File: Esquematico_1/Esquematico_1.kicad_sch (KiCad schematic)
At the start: 0 parts

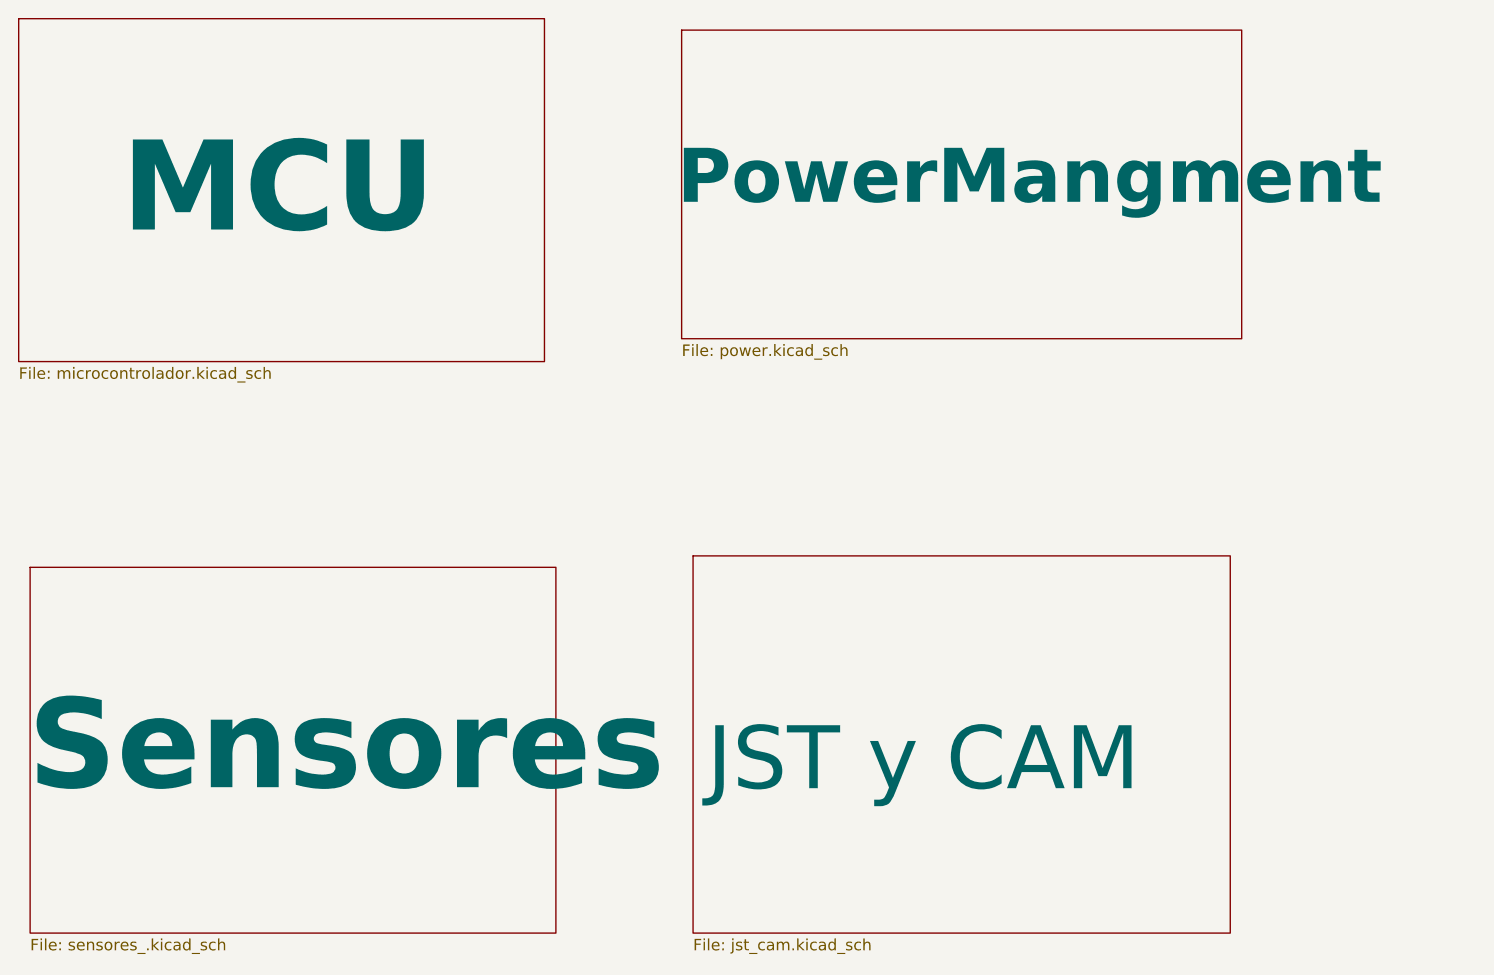
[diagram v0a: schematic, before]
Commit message: Update llamada
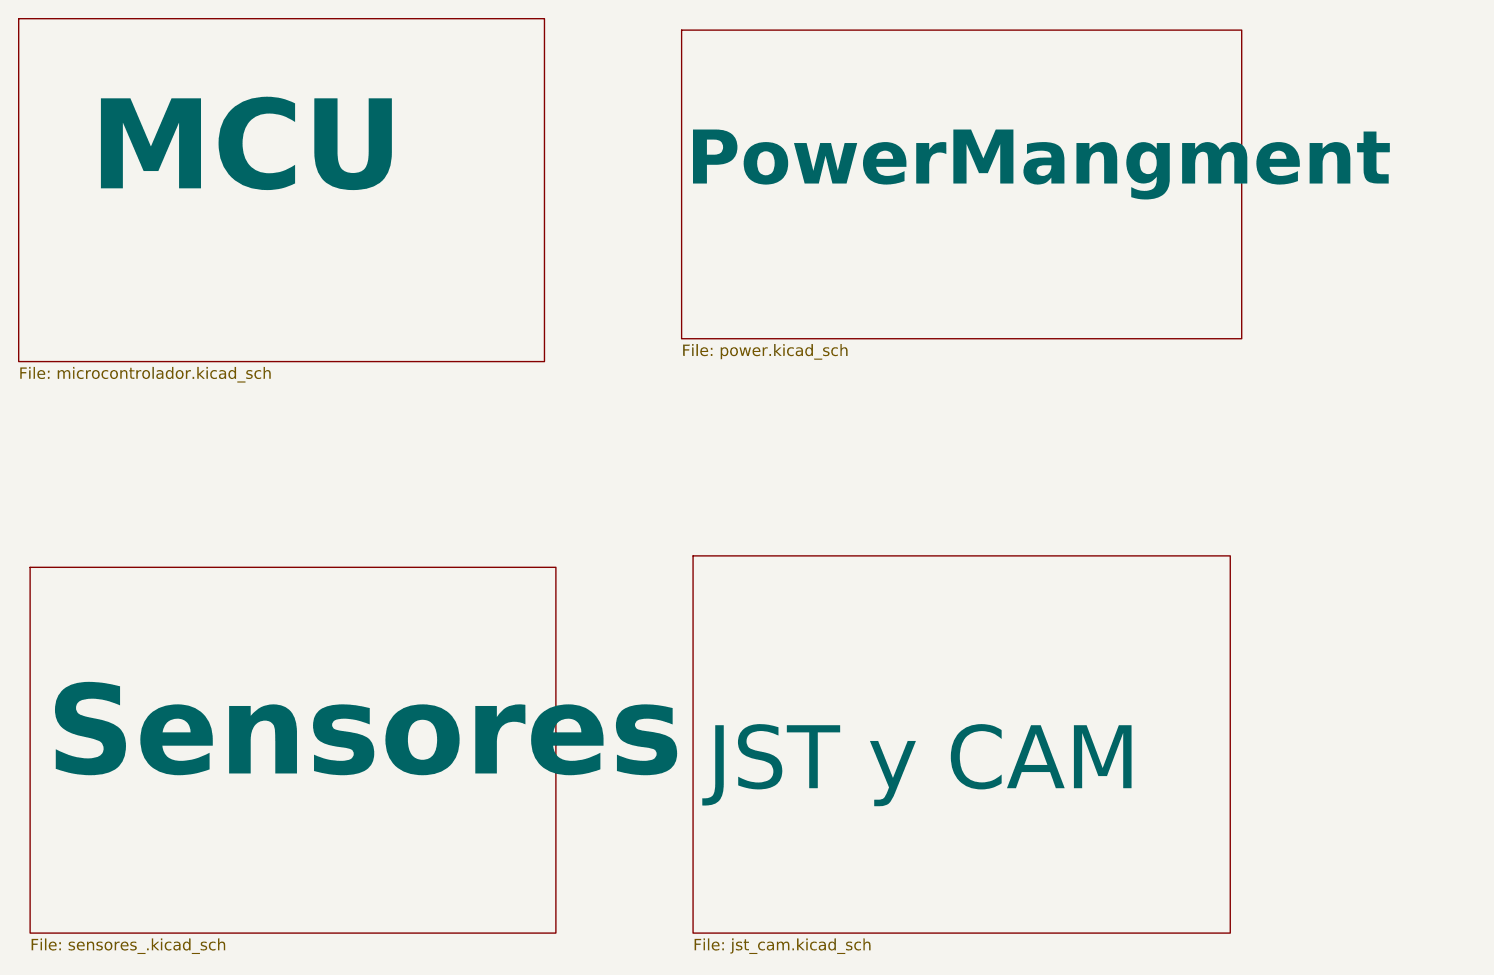
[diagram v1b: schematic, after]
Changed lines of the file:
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@@
 		)
 		(property "Sheetname" "PowerMangment"
-			(at 101.092 46.482 0)
+			(at 102.108 44.45 0)
 			(effects
 				(font
@@
 		)
 		(property "Sheetname" "Sensores"
-			(at 28.956 112.014 0)
+			(at 30.988 110.49 0)
 			(effects
 				(font
@@
 		)
 		(property "Sheetname" "MCU"
-			(at 39.37 44.196 0)
+			(at 35.814 39.624 0)
 			(effects
 				(font

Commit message: Update footprint sw rst
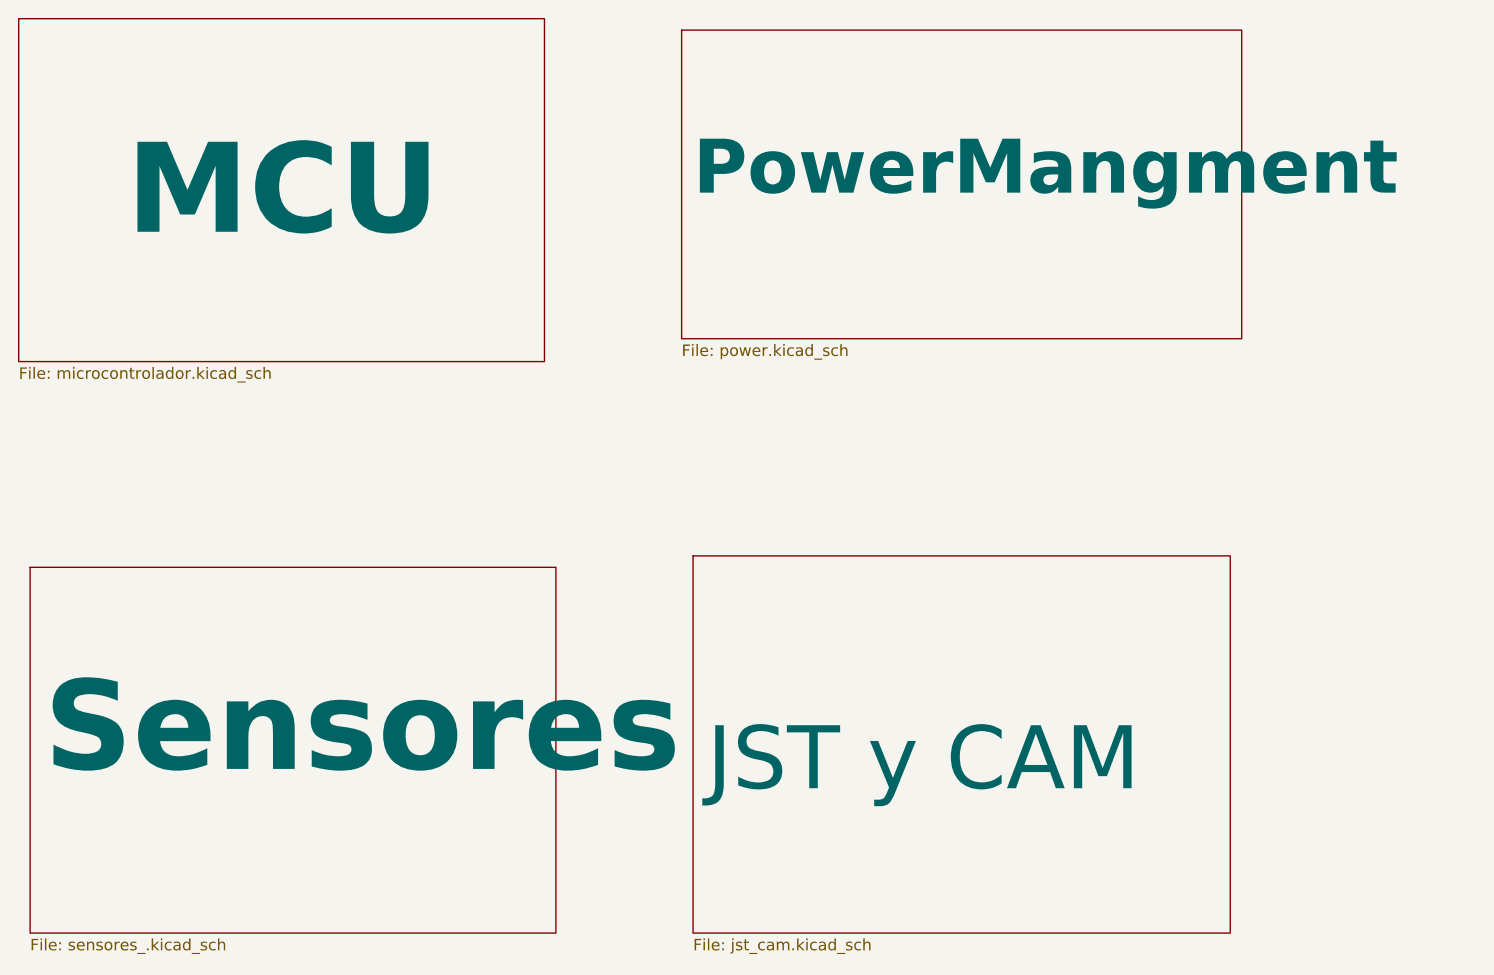
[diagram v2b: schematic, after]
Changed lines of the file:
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@@
 		)
 		(property "Sheetname" "PowerMangment"
-			(at 102.108 44.45 0)
+			(at 102.87 45.466 0)
 			(effects
 				(font
@@
 		)
 		(property "Sheetname" "Sensores"
-			(at 30.988 110.49 0)
+			(at 30.734 109.982 0)
 			(effects
 				(font
@@
 		)
 		(property "Sheetname" "MCU"
-			(at 35.814 39.624 0)
+			(at 39.878 44.45 0)
 			(effects
 				(font
